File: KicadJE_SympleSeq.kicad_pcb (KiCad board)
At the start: 2 copper layers, 80 x 100 mm, 96 parts, among them J101 CV-Out, J102 Reset + Step, J103 CV-G8_Mod1, J104 CV-G8_Mod2, J105 Hold_Rst, J106 G8-Out, J107 Reset + Step 1-4, J108 Reset + Step 5-8, J109 CV-G8_Base, J201 clk_in, J202 clk_out, J203 Hold, J204 Reset, J205 Slave clock sel, P201 HEADER_2x5_Doepfer, SW301 SW_SPDT, SW302 SW_SPDT, SW303 SW_SPDT, SW304 SW_SPDT, U101 TL082, U201 LM555, U202 4017

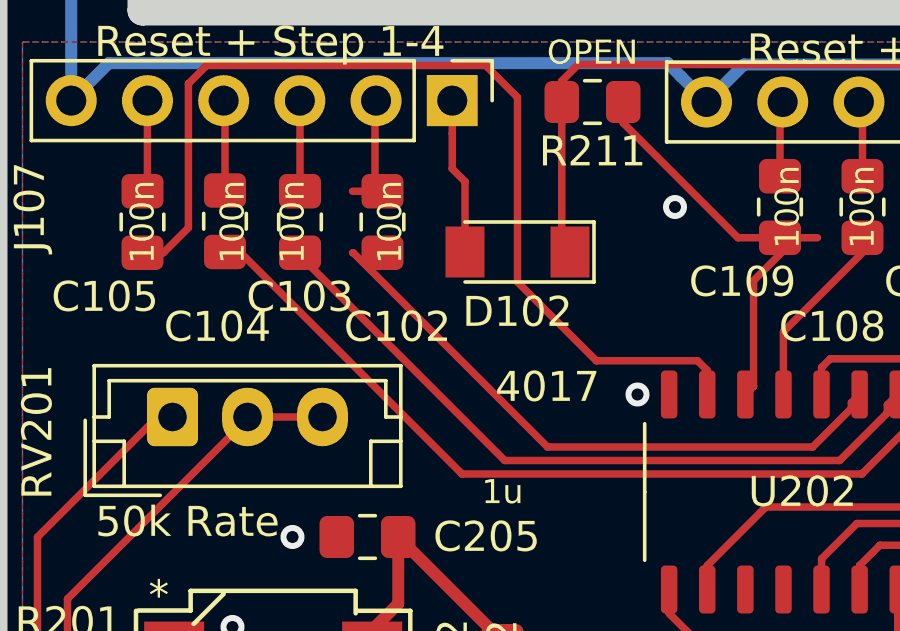
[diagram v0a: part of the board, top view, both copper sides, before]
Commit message: Unconnected fix
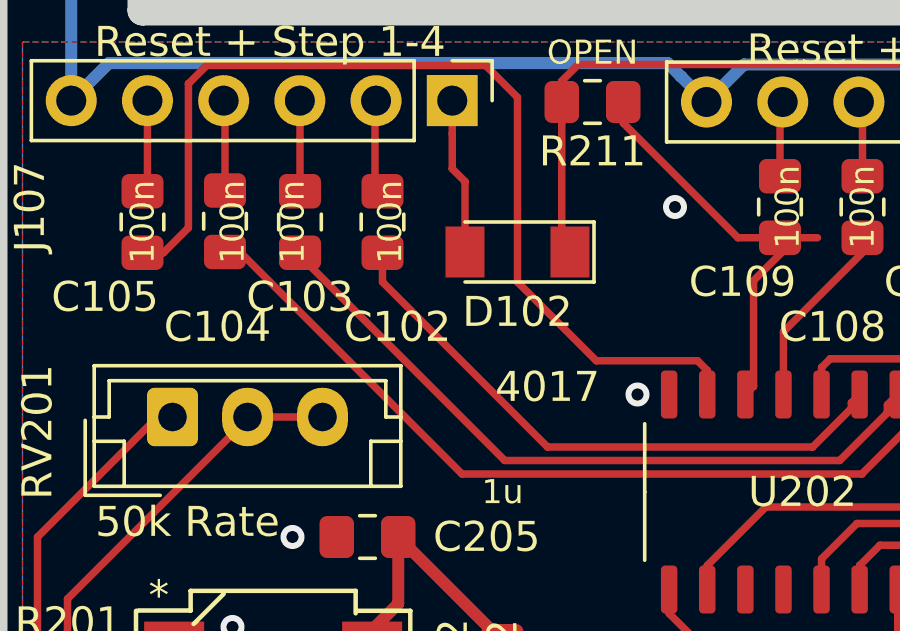
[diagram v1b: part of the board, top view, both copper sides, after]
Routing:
- net Net-(C102-Pad2): track 3.64 -> 2.78 mm
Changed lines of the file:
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@@
     (thickness 1.6)
     (drawings 27)
-    (tracks 634)
+    (tracks 632)
     (zones 0)
     (modules 96)
@@
   (segment (start 130.77501 109.835466) (end 130.77501 111.604078) (width 0.25) (layer F.Cu) (net 34))
   (segment (start 130.5 109.560456) (end 130.77501 109.835466) (width 0.25) (layer F.Cu) (net 34))
-  (segment (start 112.025 106.025) (end 112 106.025) (width 0.25) (layer F.Cu) (net 35))
-  (segment (start 128.63 111.025) (end 128.63 111.209088) (width 0.25) (layer F.Cu) (net 35) (status 30))
-  (segment (start 128.63 111.209088) (end 127.339088 112.5) (width 0.25) (layer F.Cu) (net 35) (status 10))
-  (segment (start 128.905 110.75) (end 128.63 111.025) (width 0.25) (layer F.Cu) (net 35) (status 30))
+  (segment (start 113 107) (end 113 106.025) (width 0.25) (layer F.Cu) (net 35))
+  (segment (start 128.63 111.025) (end 128.63 111.209088) (width 0.25) (layer F.Cu) (net 35))
+  (segment (start 128.905 110.75) (end 128.63 111.025) (width 0.25) (layer F.Cu) (net 35))
+  (segment (start 128.63 111.209088) (end 127.339088 112.5) (width 0.25) (layer F.Cu) (net 35))
   (segment (start 127.339088 112.5) (end 118.5 112.5) (width 0.25) (layer F.Cu) (net 35))
-  (segment (start 118.5 112.5) (end 112.025 106.025) (width 0.25) (layer F.Cu) (net 35))
+  (segment (start 118.5 112.5) (end 113 107) (width 0.25) (layer F.Cu) (net 35))
   (segment (start 129.82929 111.09571) (end 129.82929 111.36212) (width 0.25) (layer F.Cu) (net 36))
   (segment (start 128.241401 112.950009) (end 117.075009 112.950009) (width 0.25) (layer F.Cu) (net 36))
@@
   (segment (start 156.874999 117.974999) (end 156.874999 114.75) (width 0.25) (layer F.Cu) (net 51))
   (segment (start 159.65 120.75) (end 156.874999 117.974999) (width 0.25) (layer F.Cu) (net 51))
-  (segment (start 112.5 103.975) (end 112 103.975) (width 0.25) (layer F.Cu) (net 52) (status 10))
-  (segment (start 112.75 103.725) (end 112.5 103.975) (width 0.25) (layer F.Cu) (net 52) (status 30))
   (segment (start 112.784999 100.955001) (end 112.75 100.99) (width 0.25) (layer F.Cu) (net 52) (status 30))
   (segment (start 112.75 100.99) (end 112.75 103.725) (width 0.25) (layer F.Cu) (net 52) (status 30))
